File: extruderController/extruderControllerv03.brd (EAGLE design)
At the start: 93.7 x 69.3 mm, 76 parts, among them IC1 LM1117MPX-5.0, IC2 MAX3467CPA, IC3 ATMEGA2561-16AU, IC4 ULN2003AD, J8 615016137621, Q2 PH7030L, Q3 PH7030L, Q4 PH7030L, Q5 PH7030L, Q6 PH7030L, X1 22-23-2081, X2 22-23-2081, X3 22-23-2101, X4 22-23-2051, X5 TSW-102-07-G-D, X8 22-23-2031, X9 22-23-2031

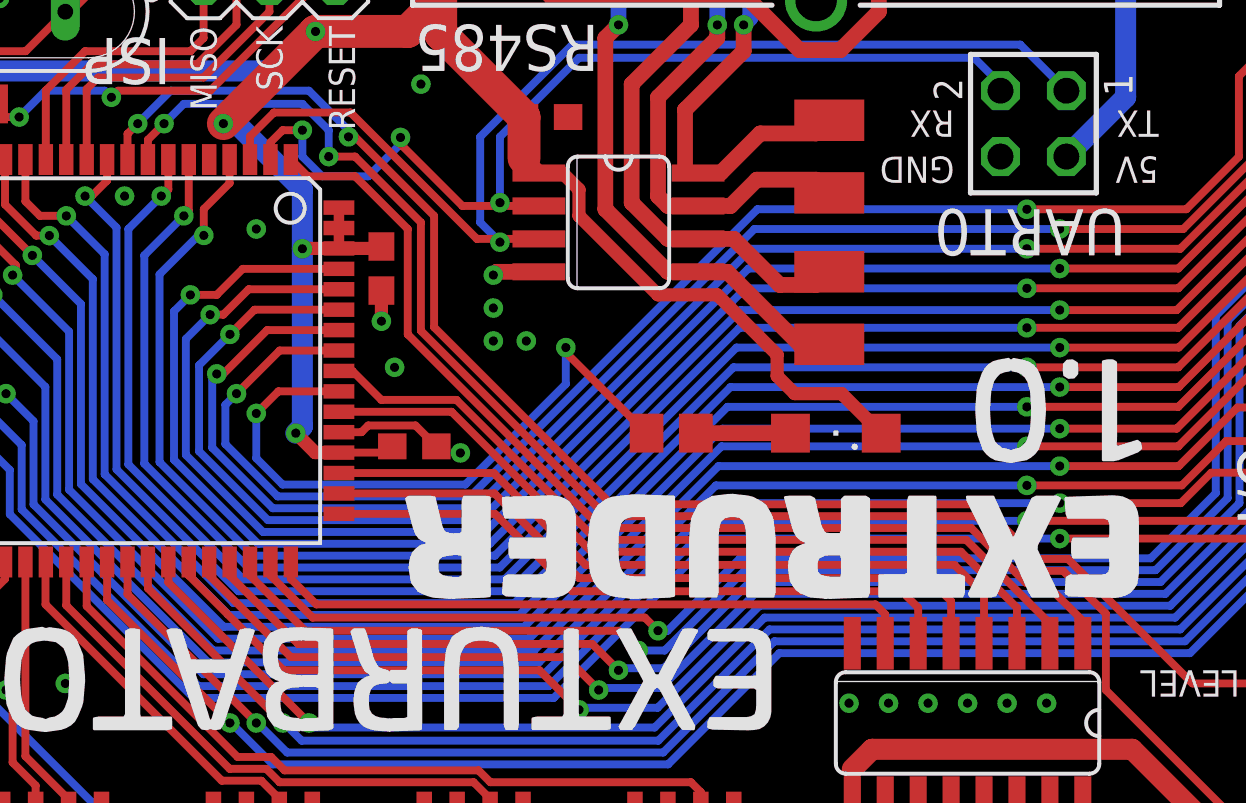
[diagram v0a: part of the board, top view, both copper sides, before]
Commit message: e
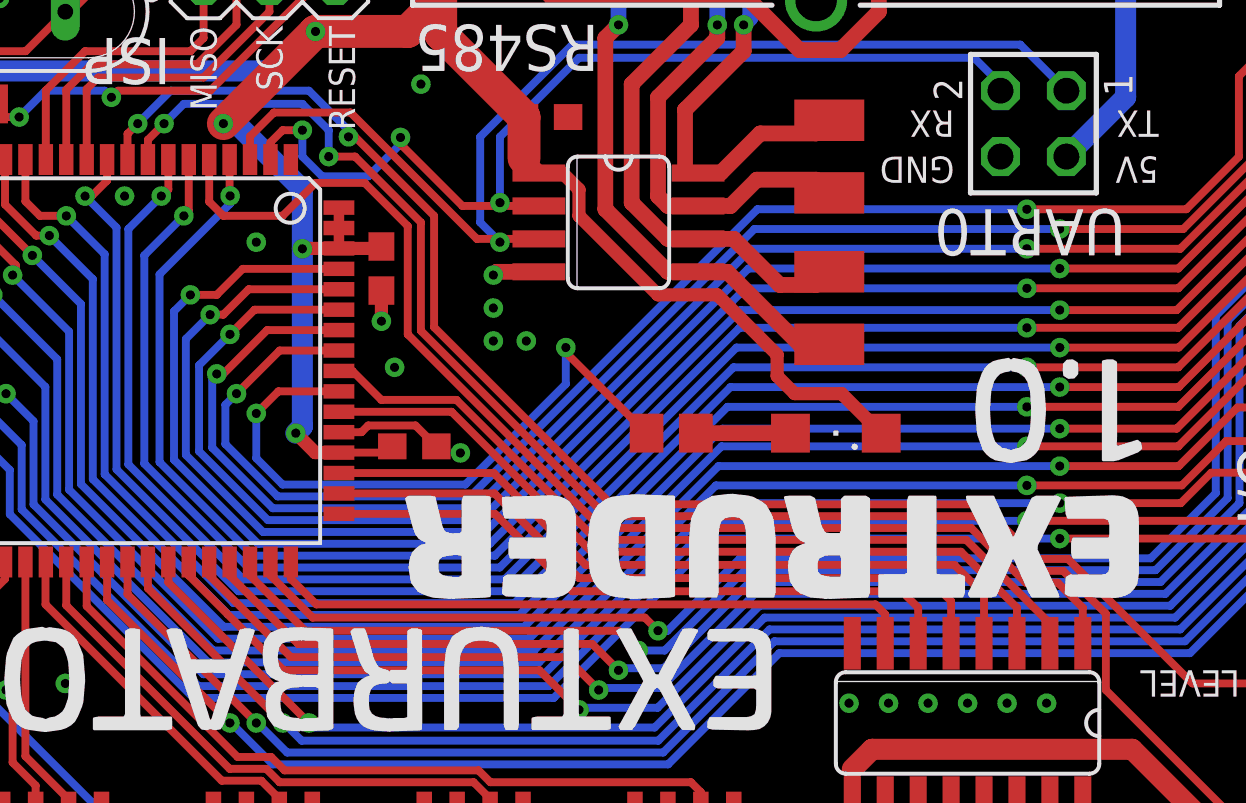
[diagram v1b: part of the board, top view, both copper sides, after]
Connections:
- net PE3: now also IC4.1
- net PG5: no longer IC4.1
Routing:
- net PE3: track 0.00 -> 46.7 mm
- net PG5: track 41.3 -> 0.00 mm
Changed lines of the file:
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@@
 <layers>
 <layer number="1" name="Top" color="4" fill="1" visible="yes" active="yes"/>
-<layer number="16" name="Bottom" color="1" fill="1" visible="no" active="yes"/>
+<layer number="16" name="Bottom" color="1" fill="1" visible="yes" active="yes"/>
 <layer number="17" name="Pads" color="2" fill="1" visible="yes" active="yes"/>
 <layer number="18" name="Vias" color="2" fill="1" visible="yes" active="yes"/>
@@
 <via x="37.592" y="44.45" extent="1-16" drill="0.35"/>
 <via x="31.75" y="38.608" extent="1-16" drill="0.35"/>
-<via x="42.672" y="43.18" extent="1-16" drill="0.35"/>
+<via x="42.672" y="42.672" extent="1-16" drill="0.35"/>
 <via x="28.448" y="26.416" extent="1-16" drill="0.35"/>
 <via x="35.306" y="25.654" extent="1-16" drill="0.35"/>
@@
 <contactref element="IC3" pad="4"/>
 <contactref element="J3" pad="7"/>
-<via x="40.64761875" y="42.93361875" extent="1-16" drill="0.35"/>
+<via x="41.66361875" y="44.45761875" extent="1-16" drill="0.35"/>
 <wire x1="51.87166875" y1="30.5816" x2="42.551" y2="30.5816" width="0.3048" layer="16"/>
-<wire x1="40.64761875" y1="42.93361875" x2="40.44370625" y2="42.93361875" width="0.3048" layer="16"/>
-<wire x1="40.44370625" y1="42.93361875" x2="38.941" y2="41.4309125" width="0.3048" layer="16"/>
+<wire x1="41.66361875" y1="44.45761875" x2="41.66361875" y2="44.15353125" width="0.3048" layer="16"/>
+<wire x1="41.66361875" y1="44.15353125" x2="38.941" y2="41.4309125" width="0.3048" layer="16"/>
 <wire x1="38.941" y1="41.4309125" x2="38.941" y2="34.1916" width="0.3048" layer="16"/>
 <wire x1="38.941" y1="34.1916" x2="42.551" y2="30.5816" width="0.3048" layer="16"/>
@@
 <wire x1="83.0834" y1="45.72753125" x2="83.0834" y2="44.96553125" width="0.3048" layer="1"/>
 <wire x1="83.0834" y1="44.96553125" x2="78.17086875" y2="40.053" width="0.3048" layer="1"/>
-<wire x1="41.6433" y1="45.8597" x2="41.6433" y2="44.9453" width="0.3048" layer="1"/>
-<wire x1="41.6433" y1="44.9453" x2="40.64761875" y2="43.94961875" width="0.3048" layer="1"/>
-<wire x1="40.64761875" y1="43.94961875" x2="40.64761875" y2="42.93361875" width="0.3048" layer="1"/>
+<wire x1="41.6433" y1="45.8597" x2="41.6433" y2="44.4779375" width="0.3048" layer="1"/>
+<wire x1="41.6433" y1="44.4779375" x2="41.66361875" y2="44.45761875" width="0.3048" layer="1"/>
 </signal>
 <signal name="PE1">
@@
 <signal name="PG5">
 <contactref element="IC3" pad="1"/>
-<wire x1="48.514" y1="39.116" x2="55.9816" y2="31.6484" width="0.3048" layer="1"/>
-<wire x1="48.514" y1="39.116" x2="48.514" y2="43.18" width="0.3048" layer="1"/>
-<wire x1="48.514" y1="43.18" x2="46.482" y2="45.212" width="0.3048" layer="1"/>
-<wire x1="44.6532" y1="45.212" x2="44.0055" y2="45.8597" width="0.3048" layer="1"/>
-<wire x1="46.482" y1="45.212" x2="44.6532" y2="45.212" width="0.3048" layer="1"/>
-<contactref element="IC4" pad="1"/>
-<wire x1="72.35003125" y1="29.5402" x2="73.0758" y2="29.5402" width="0.3048" layer="1"/>
-<wire x1="73.0758" y1="29.5402" x2="74.676" y2="27.94" width="0.3048" layer="1"/>
-<wire x1="70.24183125" y1="31.6484" x2="72.35003125" y2="29.5402" width="0.3048" layer="1"/>
-<wire x1="74.676" y1="27.94" x2="74.676" y2="27.3304" width="0.3048" layer="1"/>
-<wire x1="74.676" y1="27.3304" x2="74.549" y2="27.2034" width="0.3048" layer="1"/>
-<wire x1="55.9816" y1="31.6484" x2="70.24183125" y2="31.6484" width="0.3048" layer="1"/>
 </signal>
 <signal name="PA4">
@@
 <signal name="PE3">
 <contactref element="IC3" pad="5"/>
+<contactref element="IC4" pad="1"/>
+<wire x1="40.8559" y1="45.8597" x2="40.8559" y2="44.2341" width="0.3048" layer="1"/>
+<wire x1="40.8559" y1="44.2341" x2="41.402" y2="43.688" width="0.3048" layer="1"/>
+<wire x1="41.402" y1="43.688" x2="43.688" y2="43.688" width="0.3048" layer="1"/>
+<wire x1="43.688" y1="43.688" x2="44.958" y2="44.958" width="0.3048" layer="1"/>
+<wire x1="44.958" y1="44.958" x2="46.85141875" y2="44.958" width="0.3048" layer="1"/>
+<wire x1="48.514" y1="39.116" x2="55.9816" y2="31.6484" width="0.3048" layer="1"/>
+<wire x1="70.24183125" y1="31.6484" x2="72.35003125" y2="29.5402" width="0.3048" layer="1"/>
+<wire x1="72.35003125" y1="29.5402" x2="73.5838" y2="29.5402" width="0.3048" layer="1"/>
+<wire x1="55.9816" y1="31.6484" x2="70.24183125" y2="31.6484" width="0.3048" layer="1"/>
+<wire x1="74.549" y1="28.575" x2="74.549" y2="27.2034" width="0.3048" layer="1"/>
+<wire x1="46.85141875" y1="44.958" x2="48.514" y2="43.29541875" width="0.3048" layer="1"/>
+<wire x1="48.514" y1="43.29541875" x2="48.514" y2="39.116" width="0.3048" layer="1"/>
+<wire x1="73.5838" y1="29.5402" x2="74.549" y2="28.575" width="0.3048" layer="1"/>
 </signal>
 <signal name="PE0">
